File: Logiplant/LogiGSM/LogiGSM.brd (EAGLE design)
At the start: 147.4 x 81.4 mm, 17 parts, among them IC1 7805TV, IC2 LM1117T-3.3-V

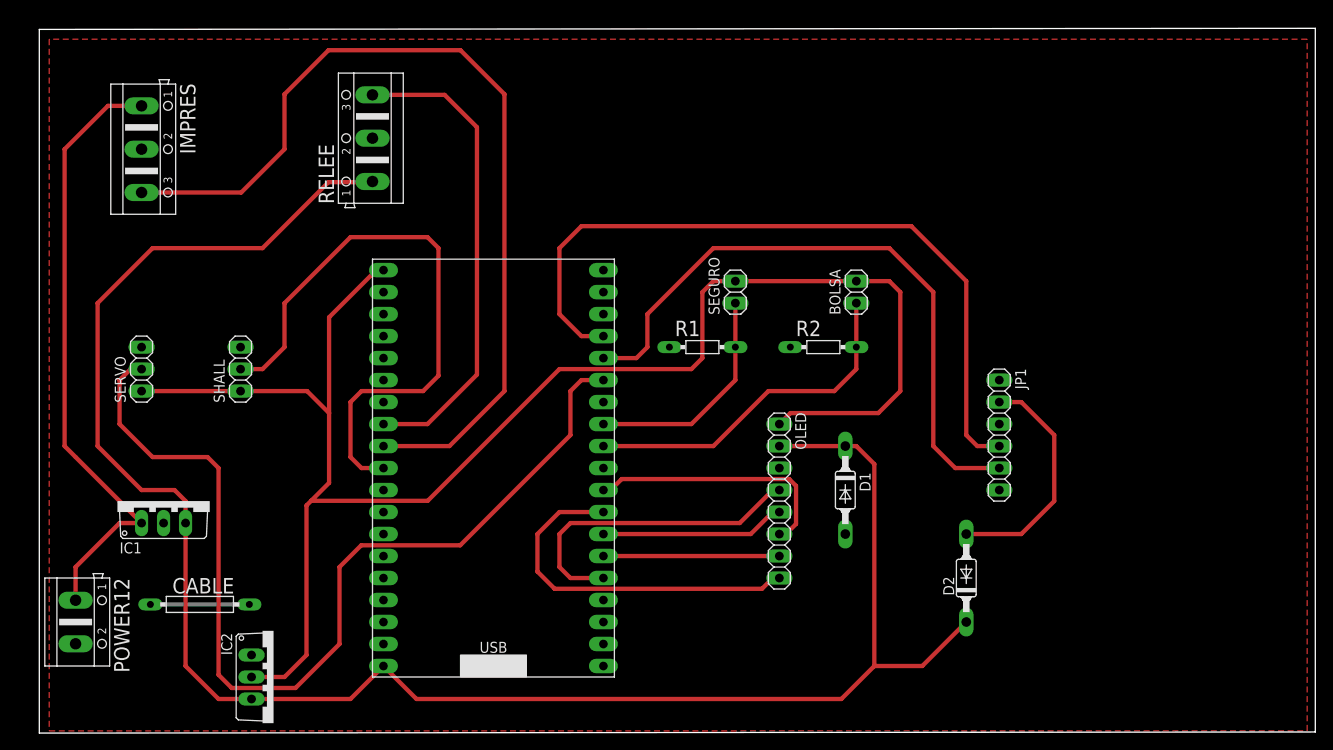
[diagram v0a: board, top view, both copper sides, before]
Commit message: Problemas con interrupcion
Problemas con interrupcion
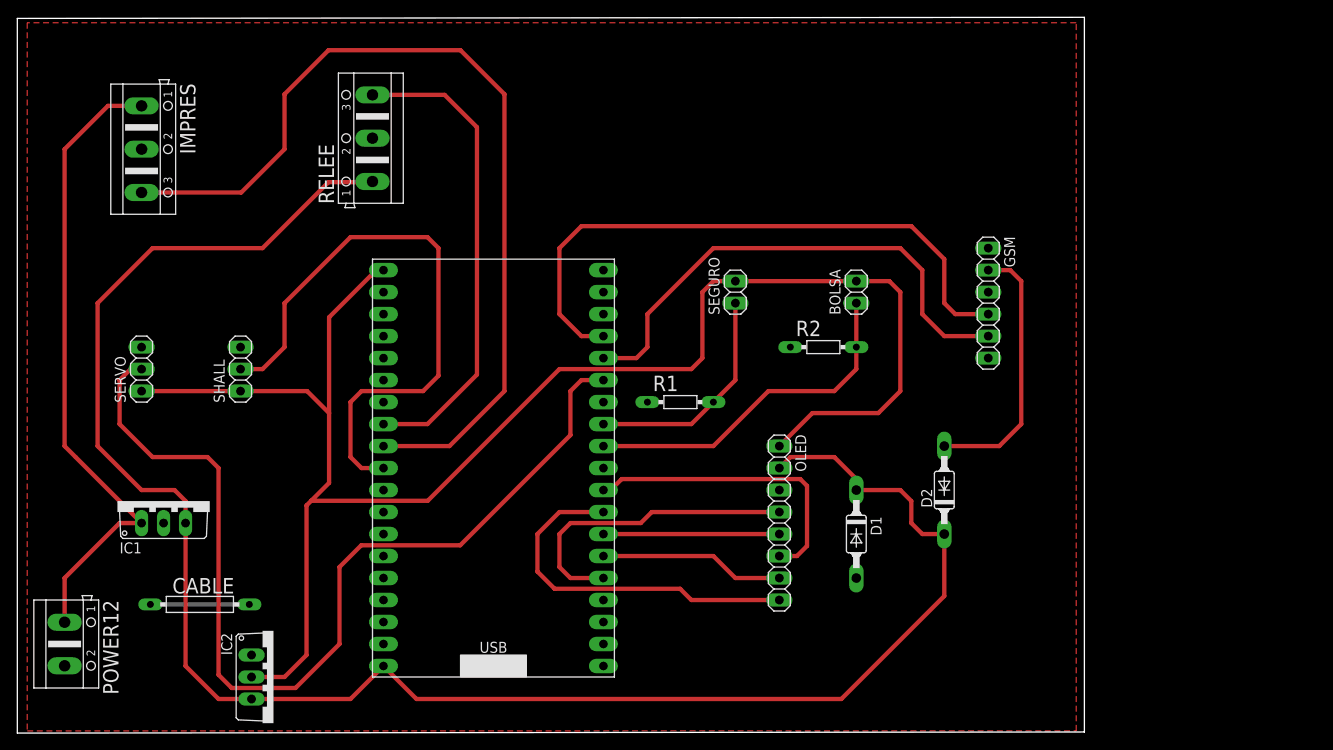
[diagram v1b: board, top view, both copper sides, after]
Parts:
- removed JP1: (no value), pinhead:1X06
- added GSM: (no value), pinhead:1X06
- moved D2 10.5 mm to (101.6, 22.9)
- moved R1 6.84 mm to (71.1, 33.0)
- moved D1 5.24 mm to (91.4, 17.8)
- moved POWER12 2.84 mm to (0.00, 5.08)
- moved OLED 2.54 mm to (82.5, 19.1)
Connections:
- net GND: now also GSM.6; no longer JP1.6
- net N$1: now also GSM.2; no longer JP1.2
- net NET: now also GSM.1; no longer JP1.1
- net RST2: now also GSM.3; no longer JP1.3
- net RXD: now also GSM.4; no longer JP1.4
- net TXD: now also GSM.5; no longer JP1.5
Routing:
- net RXD: track 86.5 -> 71.5 mm
- net TXD: track 74.1 -> 59.1 mm
- net MOSI-DATA: track 29.9 -> 35.0 mm
- net +5V: track 219.7 -> 215.9 mm
- net N$1: track 27.3 -> 30.8 mm
- net +12V: track 71.4 -> 74.5 mm
- net SCK: track 21.4 -> 20.3 mm
- net CS: track 20.3 -> 21.4 mm
- net RST: track 36.9 -> 35.9 mm
- net +3V3: track 189.3 -> 190.3 mm
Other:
- board size 147.4 x 81.4 mm -> 123.2 x 82.7 mm
